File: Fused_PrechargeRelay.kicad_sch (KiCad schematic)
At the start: 12 parts, among them K1 DE1a-12V, Q1 NMOS

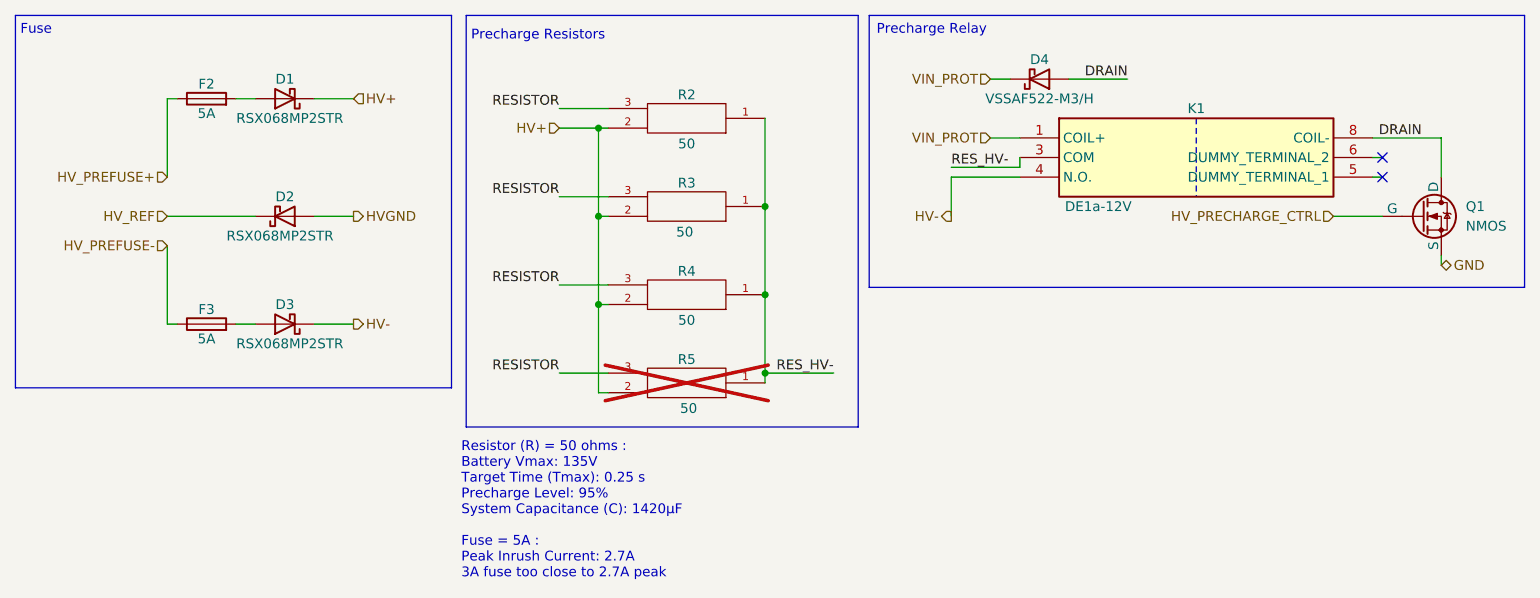
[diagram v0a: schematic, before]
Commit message: isolated precharge from fuse
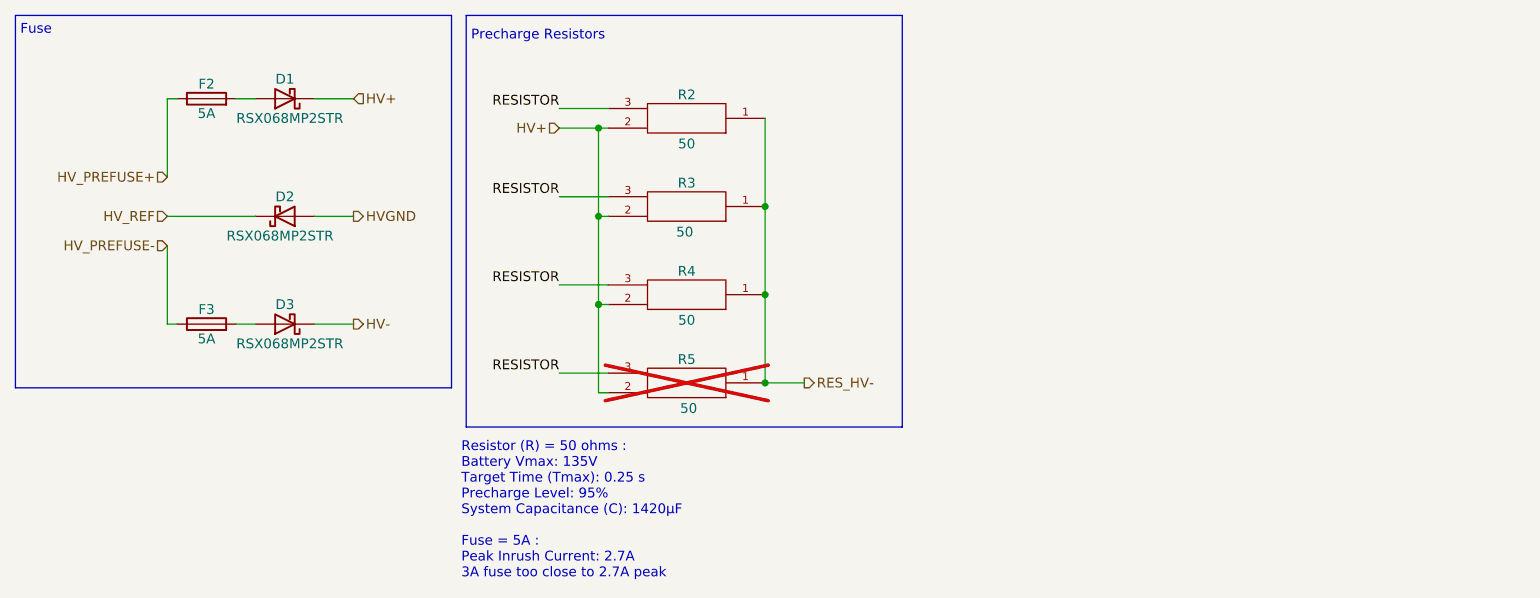
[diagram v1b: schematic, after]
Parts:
- removed D4: VSSAF522-M3/H, UTSVT-Passives:SODFL5026X125N, symbol Device:D_Schottky
- removed K1: DE1a-12V, LIB_DE1a-12V:DE1a12V, symbol DE1a-12V:DE1a-12V
- removed Q1: NMOS, ActivePrecharge-RevB:RES_PWR263S-35-3300F, symbol Simulation_SPICE:NMOS
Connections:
- no-connect marks 2 -> 0
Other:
- note removed: "Precharge Relay"
